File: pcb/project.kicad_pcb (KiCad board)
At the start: 2 copper layers, 50.8 x 76.2 mm, 11 parts, among them J1 Pi Pico Headers 1-20, J2 Pi Pico Headers 21-40, J3 12v Wall Power, J4 Reader/NeoPixel, J5 12v Door Lock, Q1 Door Switch, U1 LM2576S-5

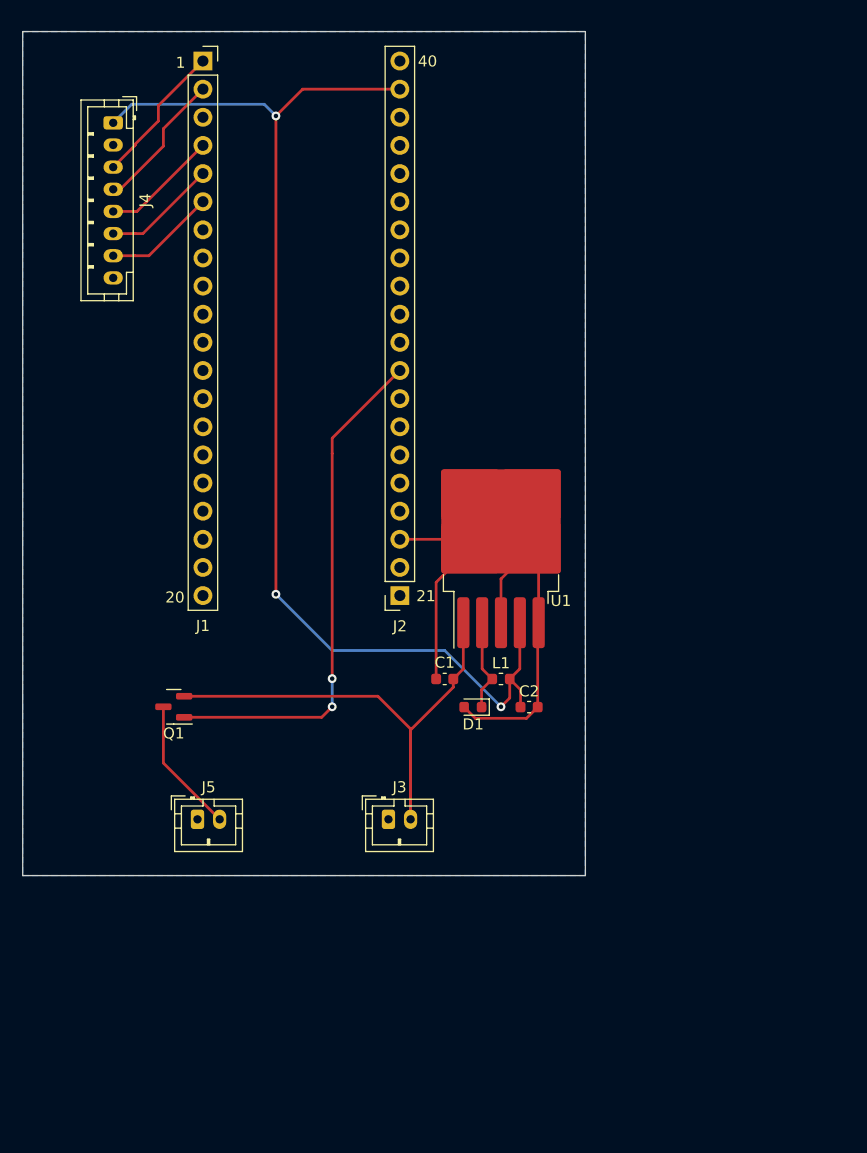
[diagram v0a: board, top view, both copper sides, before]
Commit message: Updated PCB
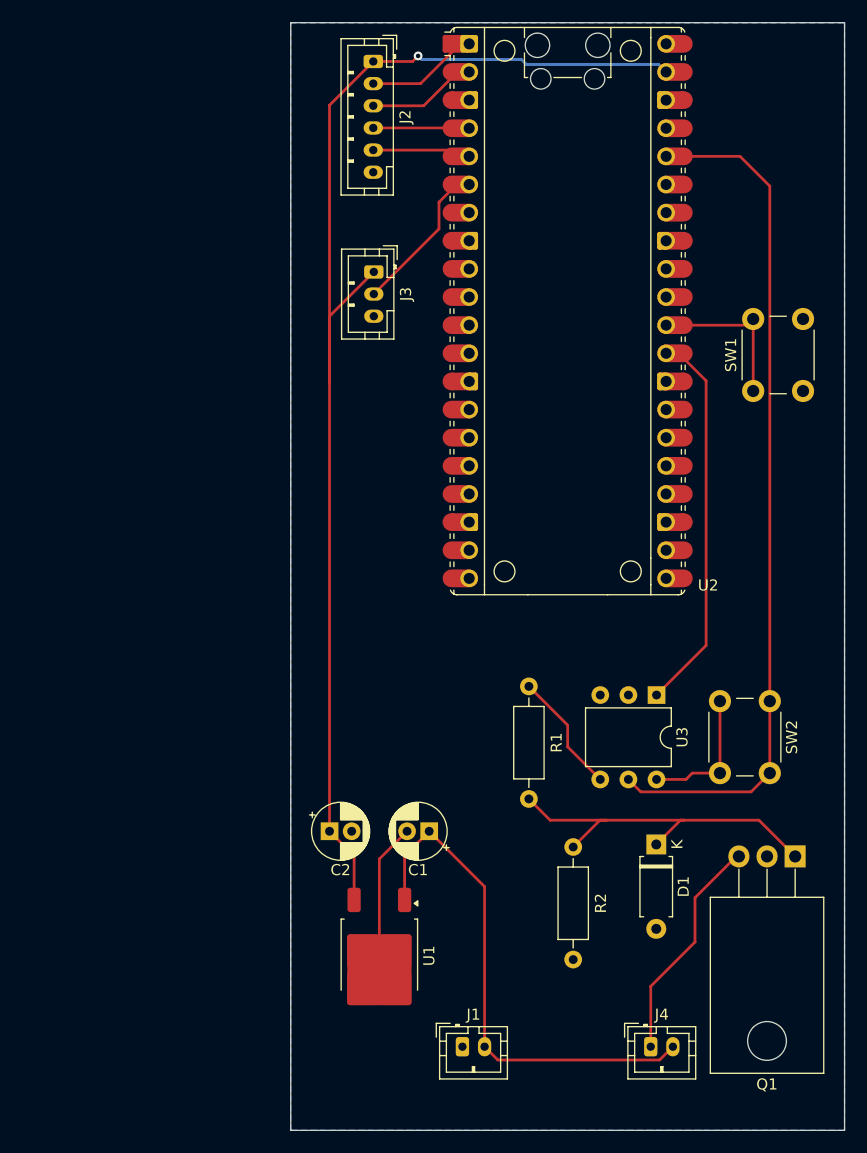
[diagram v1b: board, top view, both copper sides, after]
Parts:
- removed J5: 12v Door Lock, Connector_JST:JST_PH_B2B-PH-K_1x02_P2.00mm_Vertical
- removed L1: 100 uH, Inductor_SMD:L_0603_1608Metric
- added R1: 10, Resistor_THT:R_Axial_DIN0207_L6.3mm_D2.5mm_P10.16mm_Horizontal, F.Cu at (96.5, 120.1)
- added R2: 10k, Resistor_THT:R_Axial_DIN0207_L6.3mm_D2.5mm_P10.16mm_Horizontal, F.Cu at (100.5, 124.4)
- added SW1: SW_Push, Button_Switch_THT:SW_PUSH_6mm, F.Cu at (116.8, 83.2)
- added SW2: SW_Push, Button_Switch_THT:SW_PUSH_6mm, F.Cu at (118.2, 111.2)
- added U2: RaspberryPi_Pico_W, Module_RaspberryPi_Pico:RaspberryPi_Pico_Common, F.Cu at (100.0, 76.0)
- added U3: 4N37, Package_DIP:DIP-6_W7.62mm, F.Cu at (108.0, 110.7)
- C1: value 100uF -> 0.33uF; footprint Capacitor_SMD:C_0603_1608Metric -> Capacitor_THT:CP_Radial_D5.0mm_P2.00mm
- C2: value 1000uF -> 0.33 uF; footprint Capacitor_SMD:C_0603_1608Metric -> Capacitor_THT:CP_Radial_D5.0mm_P2.00mm
- D1: value 1N5822 -> 1N5242BTR; footprint Diode_SMD:D_0603_1608Metric -> Diode_THT:D_A-405_P7.62mm_Horizontal
- J1: value Pi Pico Headers 1-20 -> 12v Wall Power; footprint Connector_PinSocket_2.54mm:PinSocket_1x20_P2.54mm_Vertical -> Connector_JST:JST_PH_B2B-PH-K_1x02_P2.00mm_Vertical
- J2: value Pi Pico Headers 21-40 -> Reader; footprint Connector_PinSocket_2.54mm:PinSocket_1x20_P2.54mm_Vertical -> Connector_JST:JST_PH_B6B-PH-K_1x06_P2.00mm_Vertical
- J3: value 12v Wall Power -> Neopixel; footprint Connector_JST:JST_PH_B2B-PH-K_1x02_P2.00mm_Vertical -> Connector_JST:JST_PH_B3B-PH-K_1x03_P2.00mm_Vertical
- J4: value Reader/NeoPixel -> 12v Door Lock; footprint Connector_JST:JST_PH_B8B-PH-K_1x08_P2.00mm_Vertical -> Connector_JST:JST_PH_B2B-PH-K_1x02_P2.00mm_Vertical
- Q1: value Door Switch -> IRF840; footprint Package_TO_SOT_SMD:SOT-23 -> Package_TO_SOT_THT:TO-220-3_Horizontal_TabDown
- U1: value LM2576S-5 -> MC7805CDTG; footprint Package_TO_SOT_SMD:TO-263-5_TabPin3 -> Package_TO_SOT_SMD:TO-252-2
- moved J4 96.5 mm to (107.5, 142.4), turned to 0 degrees
- moved J1 92.0 mm to (90.5, 142.4)
- moved Q1 57.7 mm to (120.5, 125.3)
- moved J3 49.4 mm to (82.5, 72.5), turned to -90 degrees
- moved J2 48.3 mm to (82.5, 53.5), turned to -90 degrees
- moved U1 39.3 mm to (83.0, 134.2), turned to -90 degrees
- moved C2 21.2 mm to (78.5, 123.0)
- moved D1 20.7 mm to (108.0, 124.2), turned to -90 degrees
- moved C1 13.8 mm to (87.5, 123.0)
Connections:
- J1 pad 1: Net-(J1-Pin_1) -> GND
- J1 pad 2: Net-(J1-Pin_2) -> +12V
- J2 pad 1: unconnected-(J2-Pin_1-Pad1) -> +5V
- J2 pad 2: unconnected-(J2-Pin_2-Pad2) -> Net-(J2-Pin_2)
- J2 pad 3: GND -> Net-(J2-Pin_3)
- J2 pad 4: unconnected-(J2-Pin_4-Pad4) -> Net-(J2-Pin_4)
- J2 pad 5: unconnected-(J2-Pin_5-Pad5) -> Net-(J2-Pin_5)
- J2 pad 6: unconnected-(J2-Pin_6-Pad6) -> GND
- J3 pad 1: GND -> +5V
- J3 pad 2: +12V -> Net-(J3-Pin_2)
- J4 pad 1: +5V -> Net-(J4-Pin_1)
- J4 pad 2: GND -> +12V
- Q1 pad 1: Net-(J2-Pin_9) -> Net-(D1-K)
- Q1 pad 2: +12V -> GND
- Q1 pad 3: Net-(J5-Pin_2) -> Net-(J4-Pin_1)
- U1 pad 2: Net-(D1-K) -> GND
- U1 pad 3: GND -> +5V
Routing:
- net +3.3V: track 0.00 -> 77.4 mm
- net Net-(J2-Pin_9): track 46.7 -> 0.00 mm, vias 2 -> 0
- net GND: track 49.8 -> 13.5 mm
- net Net-(U2-GPIO22): track 0.00 -> 34.9 mm
- net Net-(D1-K): track 8.40 -> 33.6 mm
- net Net-(J4-Pin_1): track 0.00 -> 20.6 mm
- net Net-(U2-RUN): track 0.00 -> 14.6 mm
- net Net-(J3-Pin_2): track 0.00 -> 14.1 mm
- net Net-(J1-Pin_1): track 12.9 -> 0.00 mm
- net Net-(J1-Pin_2): track 12.8 -> 0.00 mm
- net Net-(SW2-Pad2): track 0.00 -> 12.5 mm
- net Net-(J5-Pin_2): track 12.3 -> 0.00 mm
- net Net-(R1-Pad2): track 0.00 -> 11.1 mm
- net Net-(J1-Pin_4): track 10.6 -> 0.00 mm
- net Net-(J1-Pin_5): track 10.3 -> 0.00 mm
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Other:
- board size 50.8 x 76.2 mm -> 50 x 100 mm
- board text removed: "1"
- board text removed: "20"
- board text removed: "21"
- board text removed: "40"
